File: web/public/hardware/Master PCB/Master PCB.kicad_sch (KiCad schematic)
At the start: 41 parts, among them J1 SWD Conn, J10 LED3, J11 LDR4, J12 LED4, J13 LED Conn, J2 OLED1, J3 OLED2, J4 5V_IN, J5 LDR1, J6 LED1, J7 LDR2, J8 LED2, J9 LDR3

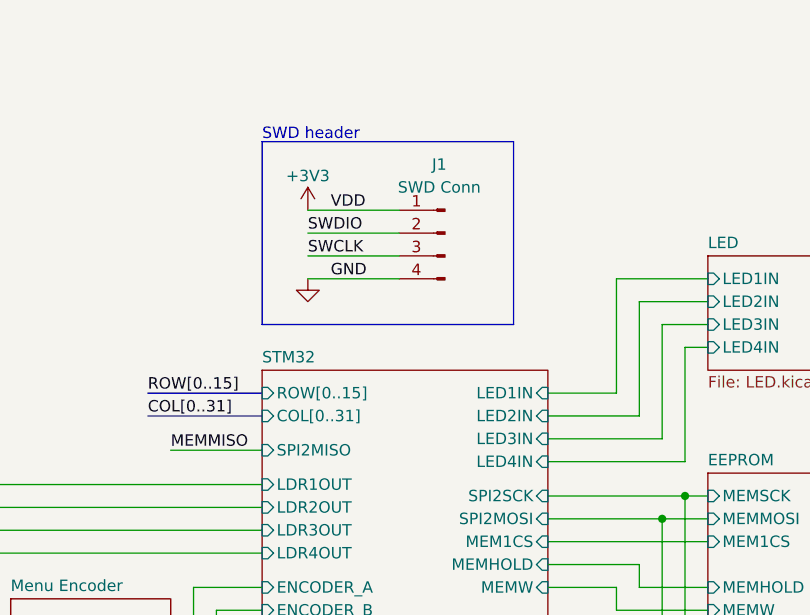
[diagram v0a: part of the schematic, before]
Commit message: Route lots
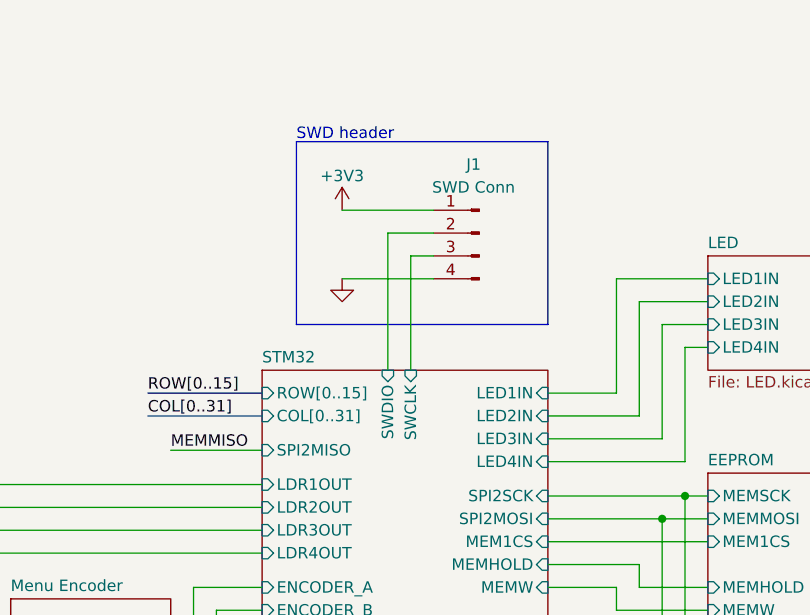
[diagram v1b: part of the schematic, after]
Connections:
- net SWCLK renamed STM32/SWCLK
- net SWDIO renamed STM32/SWDIO
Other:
- sheet STM32 ports: added SWCLK, SWDIO; removed none
- moved on the sheet: J1
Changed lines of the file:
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@@
+    (stroke (width 0) (type default))
+  )
+  (wire (pts (xy 191.77 39.37) (xy 191.77 54.61))
     (stroke (width 0) (type default))
   )
@@
     (stroke (width 0) (type default))
   )
+  (wire (pts (xy 194.31 41.91) (xy 194.31 54.61))
+    (stroke (width 0) (type default))
+  )
   (wire (pts (xy 97.79 43.18) (xy 97.79 36.83))
     (stroke (width 0) (type default))
@@
     (stroke (width 0) (type default))
   )
-  (wire (pts (xy 193.04 44.45) (xy 182.88 44.45))
+  (wire (pts (xy 196.85 44.45) (xy 186.69 44.45))
     (stroke (width 0) (type default))
   )
@@
     (stroke (width 0) (type default))
   )
+  (wire (pts (xy 196.85 39.37) (xy 191.77 39.37))
+    (stroke (width 0) (type default))
+  )
   (bus (pts (xy 49.53 49.53) (xy 49.53 52.07))
     (stroke (width 0) (type default))
@@
     (stroke (width 0) (type default))
   )
-  (wire (pts (xy 193.04 39.37) (xy 182.88 39.37))
-    (stroke (width 0) (type default))
-  )
   (wire (pts (xy 209.55 57.15) (xy 217.17 57.15))
     (stroke (width 0) (type default))
@@
     (stroke (width 0) (type default))
   )
-  (wire (pts (xy 193.04 41.91) (xy 182.88 41.91))
-    (stroke (width 0) (type default))
-  )
   (wire (pts (xy 172.72 81.28) (xy 177.8 81.28))
     (stroke (width 0) (type default))
@@
     (stroke (width 0) (type default))
   )
+  (wire (pts (xy 196.85 41.91) (xy 194.31 41.91))
+    (stroke (width 0) (type default))
+  )
   (wire (pts (xy 113.03 27.94) (xy 113.03 34.29))
     (stroke (width 0) (type default))
@@
     (stroke (width 0) (type default))
   )
-  (wire (pts (xy 193.04 36.83) (xy 182.88 36.83))
+  (wire (pts (xy 196.85 36.83) (xy 186.69 36.83))
     (stroke (width 0) (type default))
   )
@@
     (fill (type none))
   )
-  (rectangle (start 177.8 29.21) (end 205.74 49.53)
+  (rectangle (start 181.61 29.21) (end 209.55 49.53)
     (stroke (width 0) (type default))
     (fill (type none))
@@
     (effects (font (size 1.27 1.27)) (justify left bottom))
   )
-  (text "SWD header" (at 177.8 29.21 0)
+  (text "SWD header" (at 181.61 29.21 0)
     (effects (font (size 1.27 1.27)) (justify left bottom))
   )
@@
     (effects (font (size 1.27 1.27)) (justify left bottom))
   )
-  (label "SWDIO" (at 182.88 39.37 0) (fields_autoplaced)
-    (effects (font (size 1.27 1.27)) (justify left bottom))
-  )
-  (label "VDD" (at 185.42 36.83 0) (fields_autoplaced)
-    (effects (font (size 1.27 1.27)) (justify left bottom))
-  )
   (label "ROW15" (at 39.37 73.66 0) (fields_autoplaced)
     (effects (font (size 1.27 1.27)) (justify left bottom))
   )
   (label "COL18" (at 74.93 83.82 0) (fields_autoplaced)
-    (effects (font (size 1.27 1.27)) (justify left bottom))
-  )
-  (label "SWCLK" (at 182.88 41.91 0) (fields_autoplaced)
     (effects (font (size 1.27 1.27)) (justify left bottom))
   )
@@
   (label "COL[0..31]" (at 85.09 22.86 180) (fields_autoplaced)
     (effects (font (size 1.27 1.27)) (justify right bottom))
-  )
-  (label "GND" (at 185.42 44.45 0) (fields_autoplaced)
-    (effects (font (size 1.27 1.27)) (justify left bottom))
   )
   (label "ROW7" (at 39.37 48.26 0) (fields_autoplaced)
@@
     )
   )
-  (symbol (lib_id "Connector:Conn_01x04_Pin") (at 198.12 39.37 0) (mirror y) (unit 1)
-    (in_bom yes) (on_board yes) (dnp no)
-    (property "Reference" "J1" (at 197.485 31.75 0)
+  (symbol (lib_id "Connector:Conn_01x04_Pin") (at 201.93 39.37 0) (mirror y) (unit 1)
+    (in_bom yes) (on_board yes) (dnp no)
+    (property "Reference" "J1" (at 201.295 31.75 0)
       (effects (font (size 1.27 1.27)))
     )
-    (property "Value" "SWD Conn" (at 197.485 34.29 0)
+    (property "Value" "SWD Conn" (at 201.295 34.29 0)
       (effects (font (size 1.27 1.27)))
     )
-    (property "Footprint" "Connector_PinHeader_2.54mm:PinHeader_1x04_P2.54mm_Vertical" (at 198.12 39.37 0)
-      (effects (font (size 1.27 1.27)) hide)
-    )
-    (property "Datasheet" "~" (at 198.12 39.37 0)
+    (property "Footprint" "Connector_PinHeader_2.54mm:PinHeader_1x04_P2.54mm_Vertical" (at 201.93 39.37 0)
+      (effects (font (size 1.27 1.27)) hide)
+    )
+    (property "Datasheet" "~" (at 201.93 39.37 0)
       (effects (font (size 1.27 1.27)) hide)
     )
@@
     )
   )
-  (symbol (lib_id "power:GND") (at 182.88 44.45 0) (mirror y) (unit 1)
+  (symbol (lib_id "power:GND") (at 186.69 44.45 0) (mirror y) (unit 1)
     (in_bom yes) (on_board yes) (dnp no) (fields_autoplaced)
-    (property "Reference" "#PWR022" (at 182.88 50.8 0)
-      (effects (font (size 1.27 1.27)) hide)
-    )
-    (property "Value" "GND" (at 182.88 49.53 0)
-      (effects (font (size 1.27 1.27)) hide)
-    )
-    (property "Footprint" "" (at 182.88 44.45 0)
-      (effects (font (size 1.27 1.27)) hide)
-    )
-    (property "Datasheet" "" (at 182.88 44.45 0)
+    (property "Reference" "#PWR022" (at 186.69 50.8 0)
+      (effects (font (size 1.27 1.27)) hide)
+    )
+    (property "Value" "GND" (at 186.69 49.53 0)
+      (effects (font (size 1.27 1.27)) hide)
+    )
+    (property "Footprint" "" (at 186.69 44.45 0)
+      (effects (font (size 1.27 1.27)) hide)
+    )
+    (property "Datasheet" "" (at 186.69 44.45 0)
       (effects (font (size 1.27 1.27)) hide)
     )
@@
     )
   )
-  (symbol (lib_id "power:+3V3") (at 182.88 36.83 0) (mirror y) (unit 1)
-    (in_bom yes) (on_board yes) (dnp no)
-    (property "Reference" "#PWR023" (at 182.88 40.64 0)
-      (effects (font (size 1.27 1.27)) hide)
-    )
-    (property "Value" "+3V3" (at 182.88 33.02 0)
+  (symbol (lib_id "power:+3V3") (at 186.69 36.83 0) (mirror y) (unit 1)
+    (in_bom yes) (on_board yes) (dnp no)
+    (property "Reference" "#PWR023" (at 186.69 40.64 0)
+      (effects (font (size 1.27 1.27)) hide)
+    )
+    (property "Value" "+3V3" (at 186.69 33.02 0)
       (effects (font (size 1.27 1.27)))
     )
-    (property "Footprint" "" (at 182.88 36.83 0)
-      (effects (font (size 1.27 1.27)) hide)
-    )
-    (property "Datasheet" "" (at 182.88 36.83 0)
+    (property "Footprint" "" (at 186.69 36.83 0)
+      (effects (font (size 1.27 1.27)) hide)
+    )
+    (property "Datasheet" "" (at 186.69 36.83 0)
       (effects (font (size 1.27 1.27)) hide)
     )
@@
       (effects (font (size 1.27 1.27)) (justify right))
     )
+    (pin "SWDIO" input (at 191.77 54.61 90)
+      (effects (font (size 1.27 1.27)) (justify right))
+    )
+    (pin "SWCLK" input (at 194.31 54.61 90)
+      (effects (font (size 1.27 1.27)) (justify right))
+    )
